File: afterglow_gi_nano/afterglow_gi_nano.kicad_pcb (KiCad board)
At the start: 2 copper layers, 69 x 118.5 mm, 58 parts, among them J1 Conn_02x17_Odd_Even, J119 OUT GI_CONN_J119, J120 OUT GI_WPC_J120, J121 OUT GI_WPC_J121, J2 POWER_CONN, Q1 FQP30N06L, Q2 FQP30N06L, Q3 FQP30N06L, Q4 FQP30N06L, Q5 FQP30N06L, U1 74LS374, U2 L7805

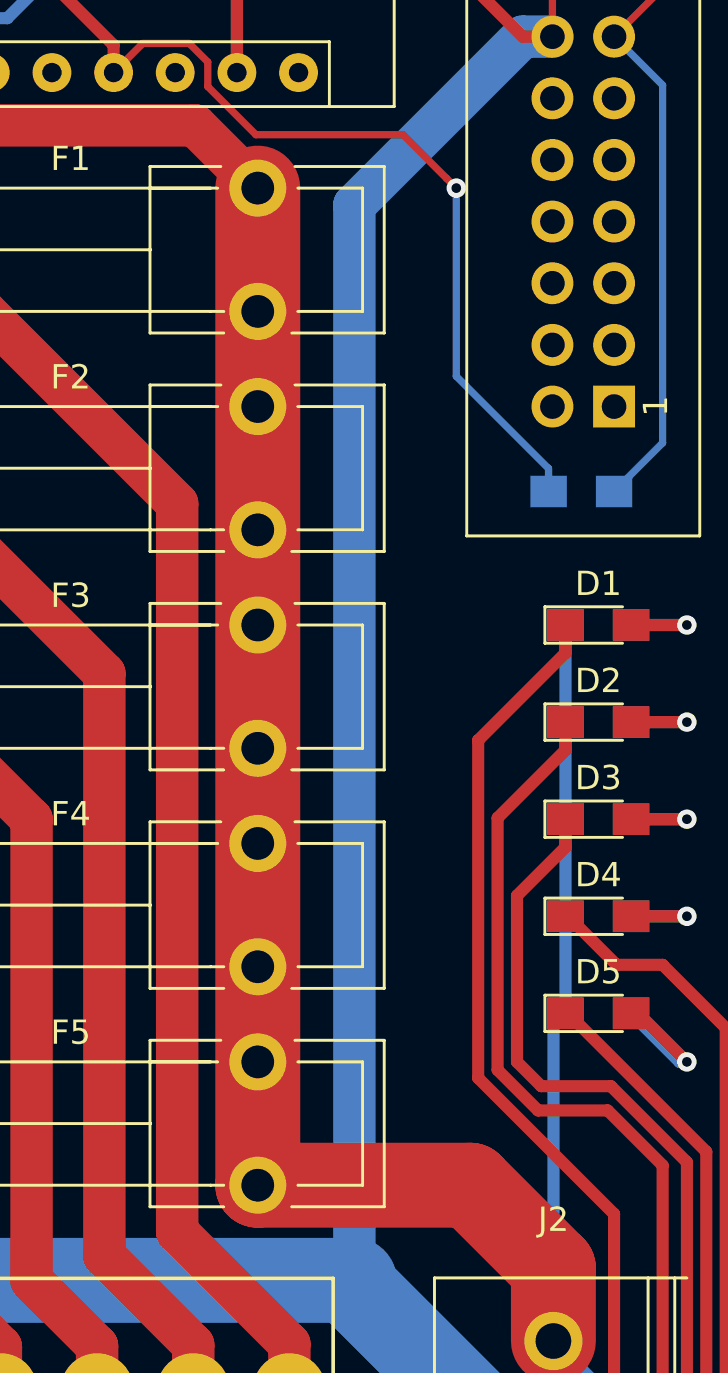
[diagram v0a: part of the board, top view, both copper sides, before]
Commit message: PCB cosmetics
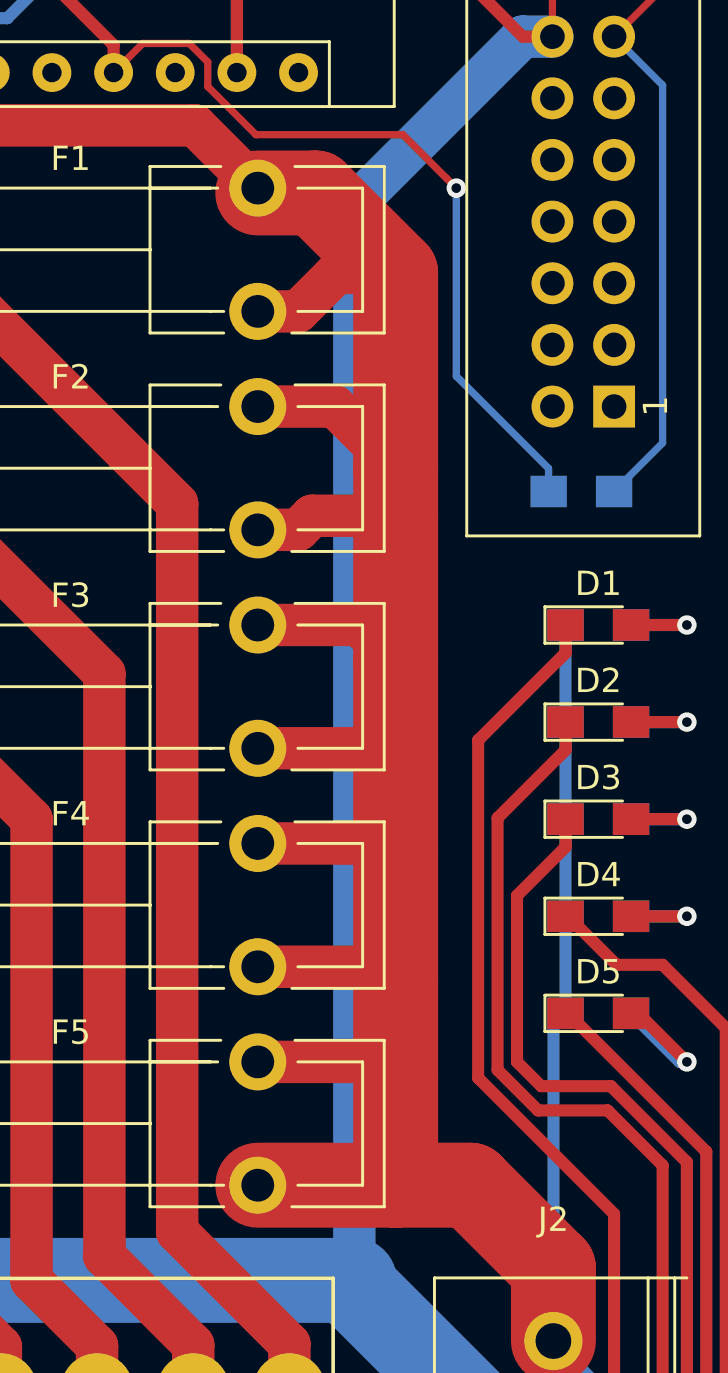
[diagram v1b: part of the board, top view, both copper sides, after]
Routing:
- net +12V: track 255.0 -> 307.3 mm
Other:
- net class 12V: clearance 0.3 -> 0.5; trace_width 0.5 -> 1.75
- net class Default: clearance 0.25 -> 0.3; trace_width 0.3 -> 0.5
- rule trace_clearance: 0.25 -> 0.3
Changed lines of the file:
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@@
     (thickness 1.6)
     (drawings 15)
-    (tracks 566)
+    (tracks 594)
     (zones 0)
     (modules 58)
@@
   )
   (setup
-    (last_trace_width 0.3)
-    (trace_clearance 0.25)
+    (last_trace_width 0.5)
+    (trace_clearance 0.3)
     (zone_clearance 0.508)
     (zone_45_only no)
@@
     (solder_mask_min_width 0.25)
     (aux_axis_origin 0 0)
-    (grid_origin 81 20.5)
+    (grid_origin 51 27.5)
     (visible_elements FFFFFF7F)
     (pcbplotparams
@@
   (net 81 "Net-(C2-Pad1)")
   (net_class Default "This is the default net class."
-    (clearance 0.25)
-    (trace_width 0.3)
+    (clearance 0.3)
+    (trace_width 0.5)
     (via_dia 0.8)
     (via_drill 0.4)
@@
   )
   (net_class 12V ""
-    (clearance 0.3)
-    (trace_width 0.5)
+    (clearance 0.5)
+    (trace_width 1.75)
     (via_dia 0.8)
     (via_drill 0.4)
@@
   (segment (start 92.580001 63.039999) (end 94.496001 63.039999) (width 0.3) (layer F.Cu) (net 2))
   (segment (start 91.38 64.24) (end 92.580001 63.039999) (width 0.3) (layer F.Cu) (net 2))
-  (segment (start 97.32 69) (end 97.32 110.08) (width 3.5) (layer F.Cu) (net 3))
   (segment (start 58.440001 36.399999) (end 59.84 35) (width 1.75) (layer F.Cu) (net 3))
   (segment (start 58.440001 62.440001) (end 58.440001 36.399999) (width 1.75) (layer F.Cu) (net 3))
@@
   (segment (start 94.735001 66.415001) (end 62.415001 66.415001) (width 1.75) (layer F.Cu) (net 3))
   (segment (start 97.32 69) (end 94.735001 66.415001) (width 1.75) (layer F.Cu) (net 3))
-  (segment (start 97.32 110.08) (end 106.08 110.08) (width 3.5) (layer F.Cu) (net 3))
   (segment (start 106.08 110.08) (end 109.5 113.5) (width 3.5) (layer F.Cu) (net 3))
   (segment (start 109.5 113.5) (end 109.5 116.5) (width 3.5) (layer F.Cu) (net 3))
@@
   (segment (start 58.440001 44.440001) (end 58.440001 36.399999) (width 0.5) (layer B.Cu) (net 3))
   (segment (start 59.5 45.5) (end 58.440001 44.440001) (width 0.5) (layer B.Cu) (net 3))
+  (segment (start 99.7 69.2) (end 97.32 69.2) (width 3.5) (layer F.Cu) (net 3))
+  (segment (start 103 72.5) (end 99.7 69.2) (width 3.5) (layer F.Cu) (net 3))
+  (segment (start 103 110.08) (end 106.08 110.08) (width 3.5) (layer F.Cu) (net 3))
+  (segment (start 97.32 110.08) (end 103 110.08) (width 3.5) (layer F.Cu) (net 3))
+  (segment (start 100.5617 72.5) (end 103 72.5) (width 1.75) (layer F.Cu) (net 3))
+  (segment (start 98.9817 74.08) (end 100.5617 72.5) (width 1.75) (layer F.Cu) (net 3))
+  (segment (start 97.32 74.08) (end 98.9817 74.08) (width 1.75) (layer F.Cu) (net 3))
+  (segment (start 100.5 78) (end 103 80.5) (width 1.75) (layer F.Cu) (net 3))
+  (segment (start 97.32 78) (end 100.5 78) (width 1.75) (layer F.Cu) (net 3))
+  (segment (start 103 80.5) (end 103 72.5) (width 3.5) (layer F.Cu) (net 3))
+  (segment (start 99.5617 82.5) (end 103 82.5) (width 1.75) (layer F.Cu) (net 3))
+  (segment (start 98.9817 83.08) (end 99.5617 82.5) (width 1.75) (layer F.Cu) (net 3))
+  (segment (start 97.32 83.08) (end 98.9817 83.08) (width 1.75) (layer F.Cu) (net 3))
+  (segment (start 103 82.5) (end 103 80.5) (width 3.5) (layer F.Cu) (net 3))
+  (segment (start 97.32 87) (end 101.5 87) (width 1.75) (layer F.Cu) (net 3))
+  (segment (start 101.5 87) (end 103 88.5) (width 1.75) (layer F.Cu) (net 3))
+  (segment (start 103 88.5) (end 103 82.5) (width 3.5) (layer F.Cu) (net 3))
+  (segment (start 102.58 92.08) (end 103 92.5) (width 1.75) (layer F.Cu) (net 3))
+  (segment (start 97.32 92.08) (end 102.58 92.08) (width 1.75) (layer F.Cu) (net 3))
+  (segment (start 103 92.5) (end 103 88.5) (width 3.5) (layer F.Cu) (net 3))
+  (segment (start 102.5 96) (end 103 96.5) (width 1.75) (layer F.Cu) (net 3))
+  (segment (start 97.32 96) (end 102.5 96) (width 1.75) (layer F.Cu) (net 3))
+  (segment (start 103 96.5) (end 103 92.5) (width 3.5) (layer F.Cu) (net 3))
+  (segment (start 102.58 101.08) (end 103 101.5) (width 1.75) (layer F.Cu) (net 3))
+  (segment (start 97.32 101.08) (end 102.58 101.08) (width 1.75) (layer F.Cu) (net 3))
+  (segment (start 103 101.5) (end 103 96.5) (width 3.5) (layer F.Cu) (net 3))
+  (segment (start 97.32 105) (end 102.5 105) (width 1.75) (layer F.Cu) (net 3))
+  (segment (start 103 110.08) (end 103 105.5) (width 3.5) (layer F.Cu) (net 3))
+  (segment (start 102.5 105) (end 103 105.5) (width 1.75) (layer F.Cu) (net 3))
+  (segment (start 103 105.5) (end 103 101.5) (width 3.5) (layer F.Cu) (net 3))
   (via (at 115 87) (size 0.8) (drill 0.4) (layers F.Cu B.Cu) (net 4))
   (segment (start 112.7 87) (end 115 87) (width 0.5) (layer F.Cu) (net 4))

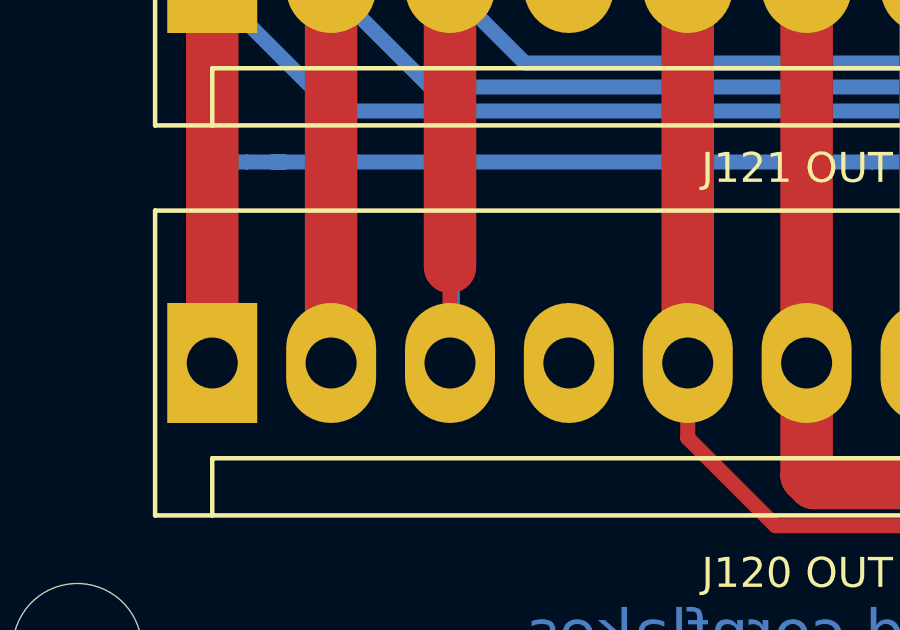
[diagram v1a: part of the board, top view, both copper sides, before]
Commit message: A PCB layout proposal
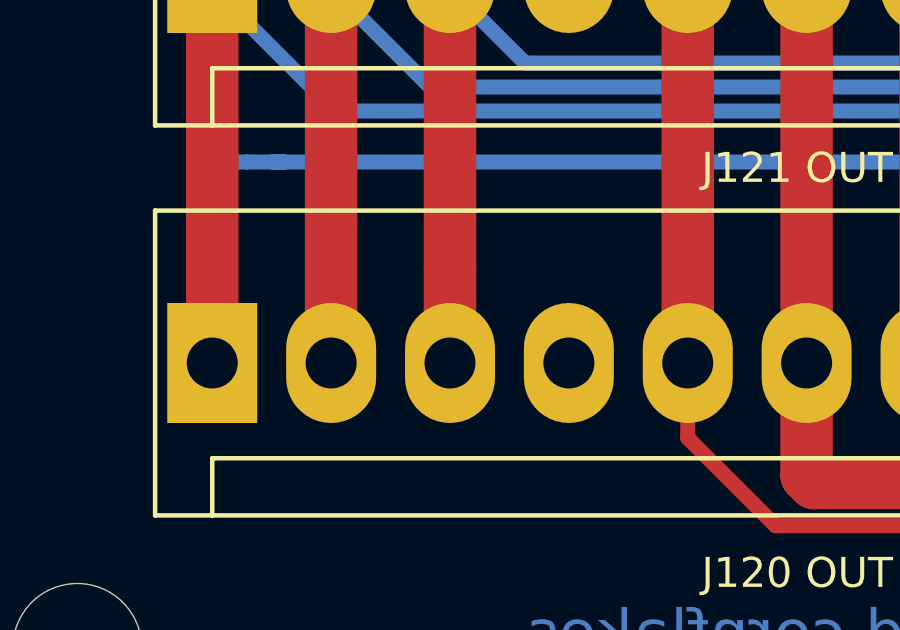
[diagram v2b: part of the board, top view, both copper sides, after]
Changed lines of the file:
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@@
-(kicad_pcb (version 20171130) (host pcbnew 5.0.1)
+(kicad_pcb (version 20171130) (host pcbnew 5.1.2)
   (general
     (thickness 1.6)
-    (drawings 15)
+    (drawings 17)
     (tracks 594)
     (zones 0)
@@
     (zone_45_only no)
     (trace_min 0.2)
-    (segment_width 0.2)
-    (edge_width 0.15)
     (via_size 0.8)
     (via_drill 0.4)
@@
     (uvia_min_size 0.2)
     (uvia_min_drill 0.1)
+    (edge_width 0.15)
+    (segment_width 0.2)
     (pcb_text_width 0.3)
     (pcb_text_size 1.5 1.5)
@@
     (uvia_dia 0.3)
     (uvia_drill 0.1)
-    (diff_pair_gap 0.5)
     (diff_pair_width 0.3)
+    (diff_pair_gap 0.5)
     (add_net +12V)
     (add_net /GI_OUT_0)
@@
       (xy 18.3 0)) (layer F.SilkS) (width 0.01))
   )
+  (dimension 69 (width 0.3) (layer F.SilkS)
+    (gr_text "69.000 mm" (at 85 159.6) (layer F.SilkS)
+      (effects (font (size 1.5 1.5) (thickness 0.3)))
+    )
+    (feature1 (pts (xy 119.5 150.5) (xy 119.5 158.086421)))
+    (feature2 (pts (xy 50.5 150.5) (xy 50.5 158.086421)))
+    (crossbar (pts (xy 50.5 157.5) (xy 119.5 157.5)))
+    (arrow1a (pts (xy 119.5 157.5) (xy 118.373496 158.086421)))
+    (arrow1b (pts (xy 119.5 157.5) (xy 118.373496 156.913579)))
+    (arrow2a (pts (xy 50.5 157.5) (xy 51.626504 158.086421)))
+    (arrow2b (pts (xy 50.5 157.5) (xy 51.626504 156.913579)))
+  )
+  (dimension 118.5 (width 0.3) (layer F.SilkS)
+    (gr_text "118.500 mm" (at 36.9 86.25 270) (layer F.SilkS)
+      (effects (font (size 1.5 1.5) (thickness 0.3)))
+    )
+    (feature1 (pts (xy 46.5 145.5) (xy 38.413579 145.5)))
+    (feature2 (pts (xy 46.5 27) (xy 38.413579 27)))
+    (crossbar (pts (xy 39 27) (xy 39 145.5)))
+    (arrow1a (pts (xy 39 145.5) (xy 38.413579 144.373496)))
+    (arrow1b (pts (xy 39 145.5) (xy 39.586421 144.373496)))
+    (arrow2a (pts (xy 39 27) (xy 38.413579 28.126504)))
+    (arrow2b (pts (xy 39 27) (xy 39.586421 28.126504)))
+  )
   (gr_text "-12V+\n" (at 117.5 119 90) (layer F.SilkS)
     (effects (font (size 1.5 1.5) (thickness 0.3)))
@@
   (segment (start 111.868616 106) (end 115 109.131384) (width 0.5) (layer F.Cu) (net 8))
   (segment (start 108 98.15) (end 108 105) (width 0.5) (layer F.Cu) (net 8))
-  (segment (start 66.9248 128.8) (end 66.9248 132) (width 0.5) (layer F.Cu) (net 8))
   (segment (start 66.9248 119) (end 66.9248 128.8) (width 1.75) (layer F.Cu) (net 8))
   (segment (start 67 131.9248) (end 66.9248 132) (width 0.5) (layer B.Cu) (net 8))
   (segment (start 67 128) (end 67 131.9248) (width 0.5) (layer B.Cu) (net 8))
+  (segment (start 66.9248 128.8) (end 66.9248 132) (width 1.75) (layer F.Cu) (net 8))
   (via (at 115 95) (size 0.8) (drill 0.4) (layers F.Cu B.Cu) (net 9))
   (segment (start 112.7 95) (end 115 95) (width 0.5) (layer F.Cu) (net 9))
